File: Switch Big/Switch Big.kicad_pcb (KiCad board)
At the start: 2 copper layers, 97.2 x 128.4 mm, 23 parts, among them SW1 SW_SPDT, SW2 SW_SPDT, SW3 SW_SPDT, SW4 SW_SPDT, SW5 SW_SPDT

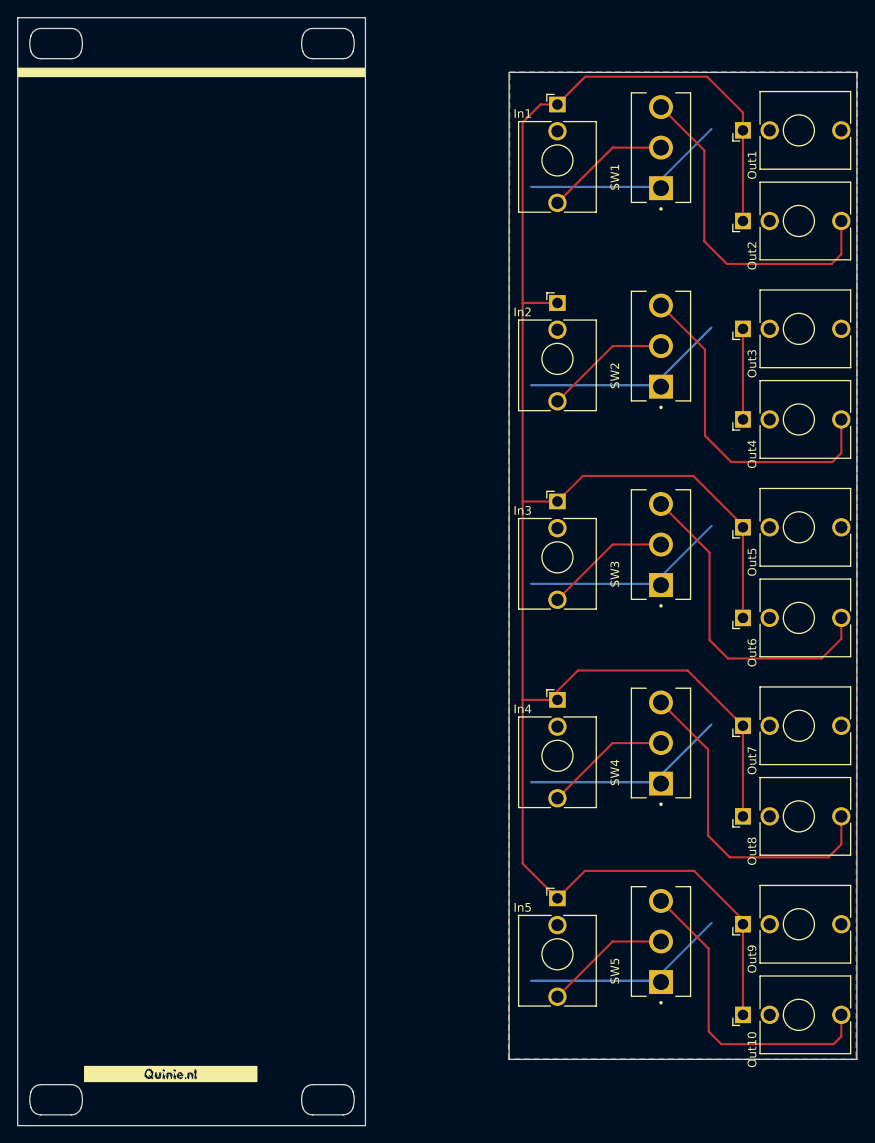
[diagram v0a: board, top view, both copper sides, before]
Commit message: GND
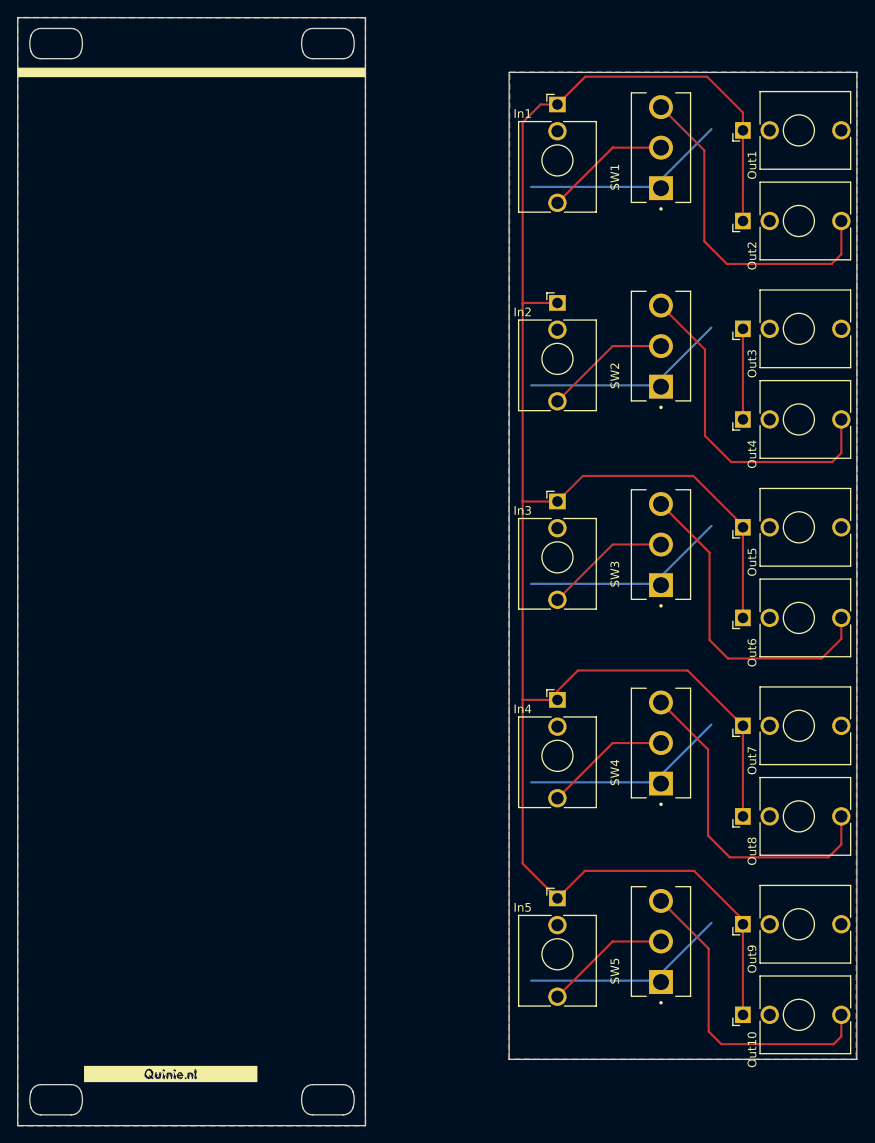
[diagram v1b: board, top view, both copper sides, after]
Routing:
- added copper zone on B.Cu, net (none)
- added copper zone on F.Cu, net (none)
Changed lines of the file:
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@@
     (connect_pads (clearance 0.5))
     (min_thickness 0.25) (filled_areas_thickness no)
-    (fill (thermal_gap 0.5) (thermal_bridge_width 0.5))
+    (fill yes (thermal_gap 0.5) (thermal_bridge_width 0.5))
     (polygon
       (pts
@@
       )
     )
+  )
+  (zone (net 0) (net_name "") (layers "F&B.Cu") (hatch edge 0.5)
+    (priority 1)
+    (connect_pads (clearance 0.5))
+    (min_thickness 0.25) (filled_areas_thickness no)
+    (fill yes (thermal_gap 0.5) (thermal_bridge_width 0.5) (island_removal_mode 1) (island_area_min 10))
+    (polygon
+      (pts
+        (xy 66.8 21.1)
+        (xy 26.5 21.075)
+        (xy 26.5 149.5)
+        (xy 66.8 149.5)
+      )
+    )
